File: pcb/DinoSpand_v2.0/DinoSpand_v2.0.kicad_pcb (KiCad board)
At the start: 2 copper layers, 70 x 59 mm, 89 parts, among them J1 Conn_01x04_Pin, J10 Conn_01x02_Pin, J11 3-794619-8, J2 Conn_01x02_Pin, J3 4-794619-6, J4 Conn_01x02_Pin, J5 Conn_01x02_Pin, J6 Conn_01x04_Pin, J7 Conn_01x02_Pin, J8 Conn_01x02_Pin, J9 Conn_01x02_Pin, K1 EE2-5NU, K2 EE2-5NU, K3 EE2-5NU, K4 EE2-5NU, Q1 DMN62D0U-7, Q2 DMN62D0U-7, Q3 DMN62D0U-7, Q4 DMN62D0U-7, U1 Oled64x128, U2 ESP32-S3-WROOM-1-N4, U3 LT1963AEST-3.3#TRPBF, U4 LT1963AEST-3.3#TRPBF

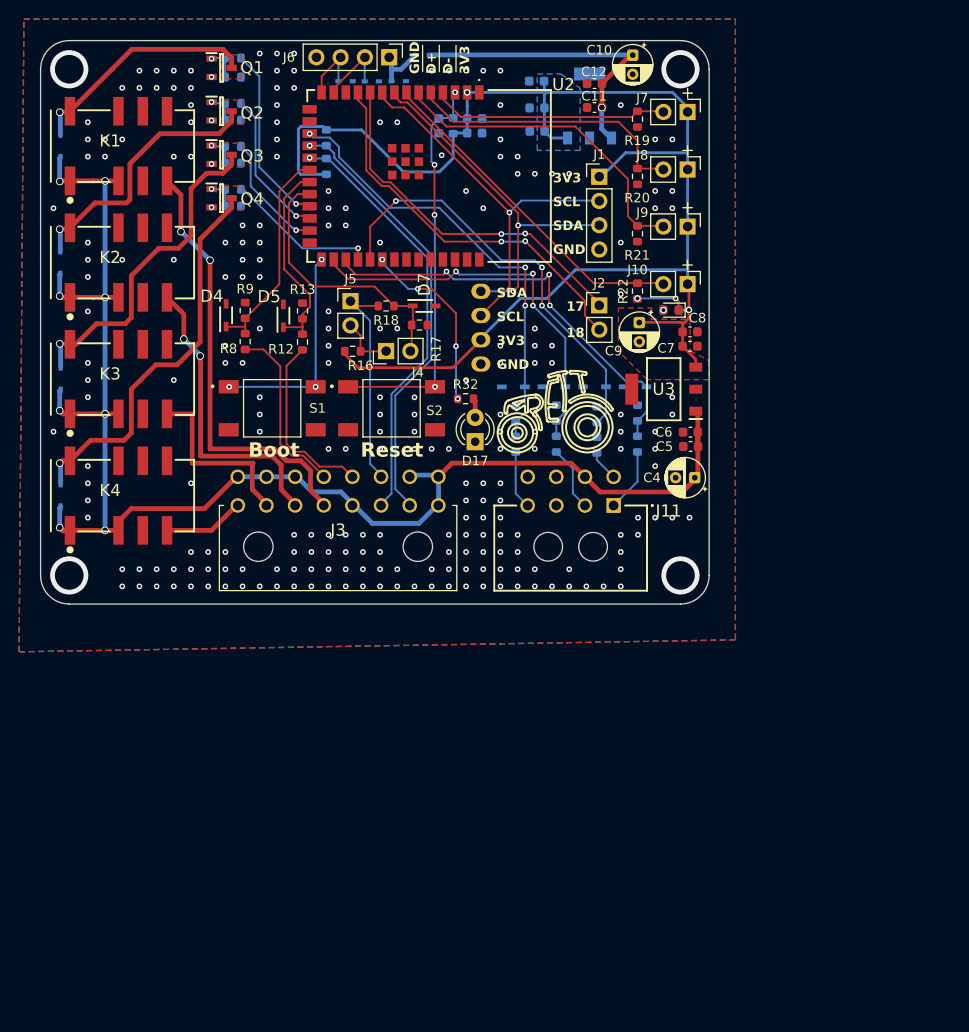
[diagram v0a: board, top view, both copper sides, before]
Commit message: pcbs update
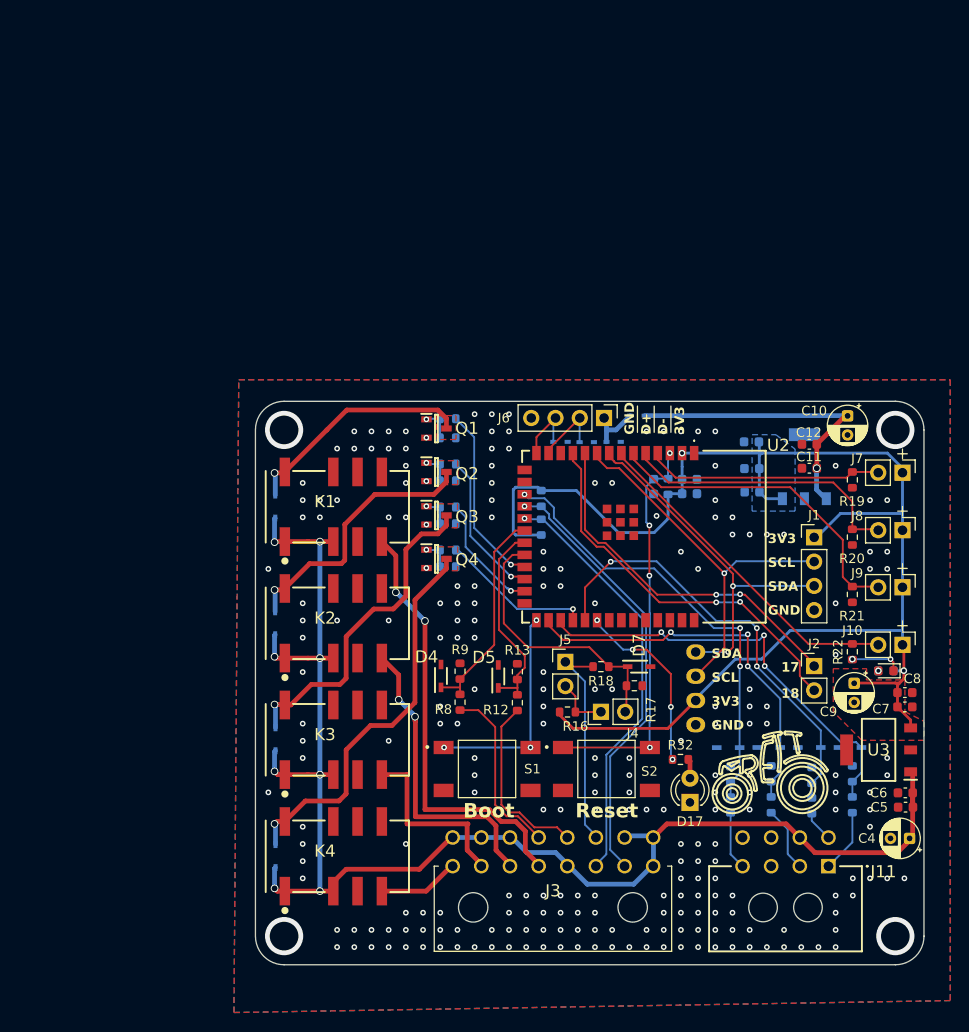
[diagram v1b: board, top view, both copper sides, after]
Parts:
- moved C1 44.0 mm to (157.9, 87.4)
- moved C2 44.0 mm to (157.9, 85.9)
- moved C3 44.0 mm to (154.2, 86.7)
- moved R1 44.0 mm to (155.7, 86.7)
- moved J5 44.0 mm to (144.9, 105.1)
- moved K3 44.0 mm to (113.6, 113.2)
- moved K4 44.0 mm to (113.6, 125.4)
- moved R16 44.0 mm to (145.2, 110.3)
- moved R18 44.0 mm to (148.7, 105.6)
- moved R4 44.0 mm to (142.4, 87.9)
- moved R7 44.0 mm to (142.4, 90.9)
- moved C11 44.0 mm to (170.5, 84.8)
- moved C14 44.0 mm to (164.5, 84.8)
- moved C5 44.0 mm to (180.6, 120.3)
- moved C6 44.0 mm to (180.5, 118.8)
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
